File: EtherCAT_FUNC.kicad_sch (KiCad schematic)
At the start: 31 parts, among them J1 axt430124, J10 Conn_01x02, J11 Conn_01x02, J12 Conn_01x02, J13 Conn_01x02, J14 Conn_01x02, J15 Conn_01x02, J16 Conn_01x02, J2 Conn_01x02, J3 Conn_01x02, J4 Conn_01x04, J8 Conn_01x03, J9 Conn_01x02, U6 ESDS314

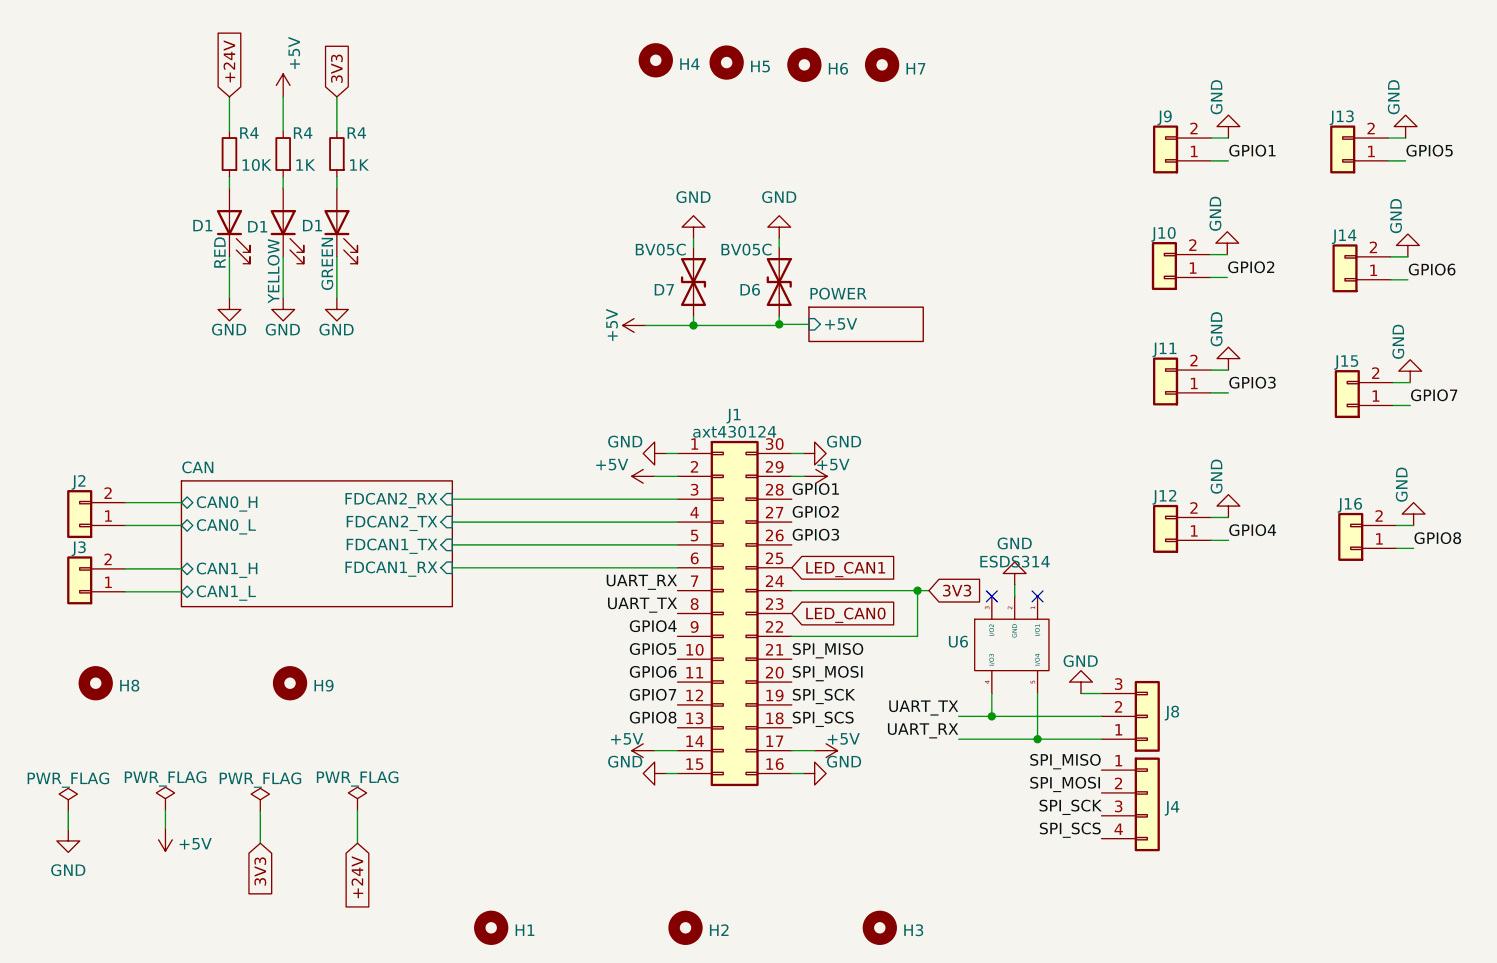
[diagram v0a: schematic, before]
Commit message: Official version
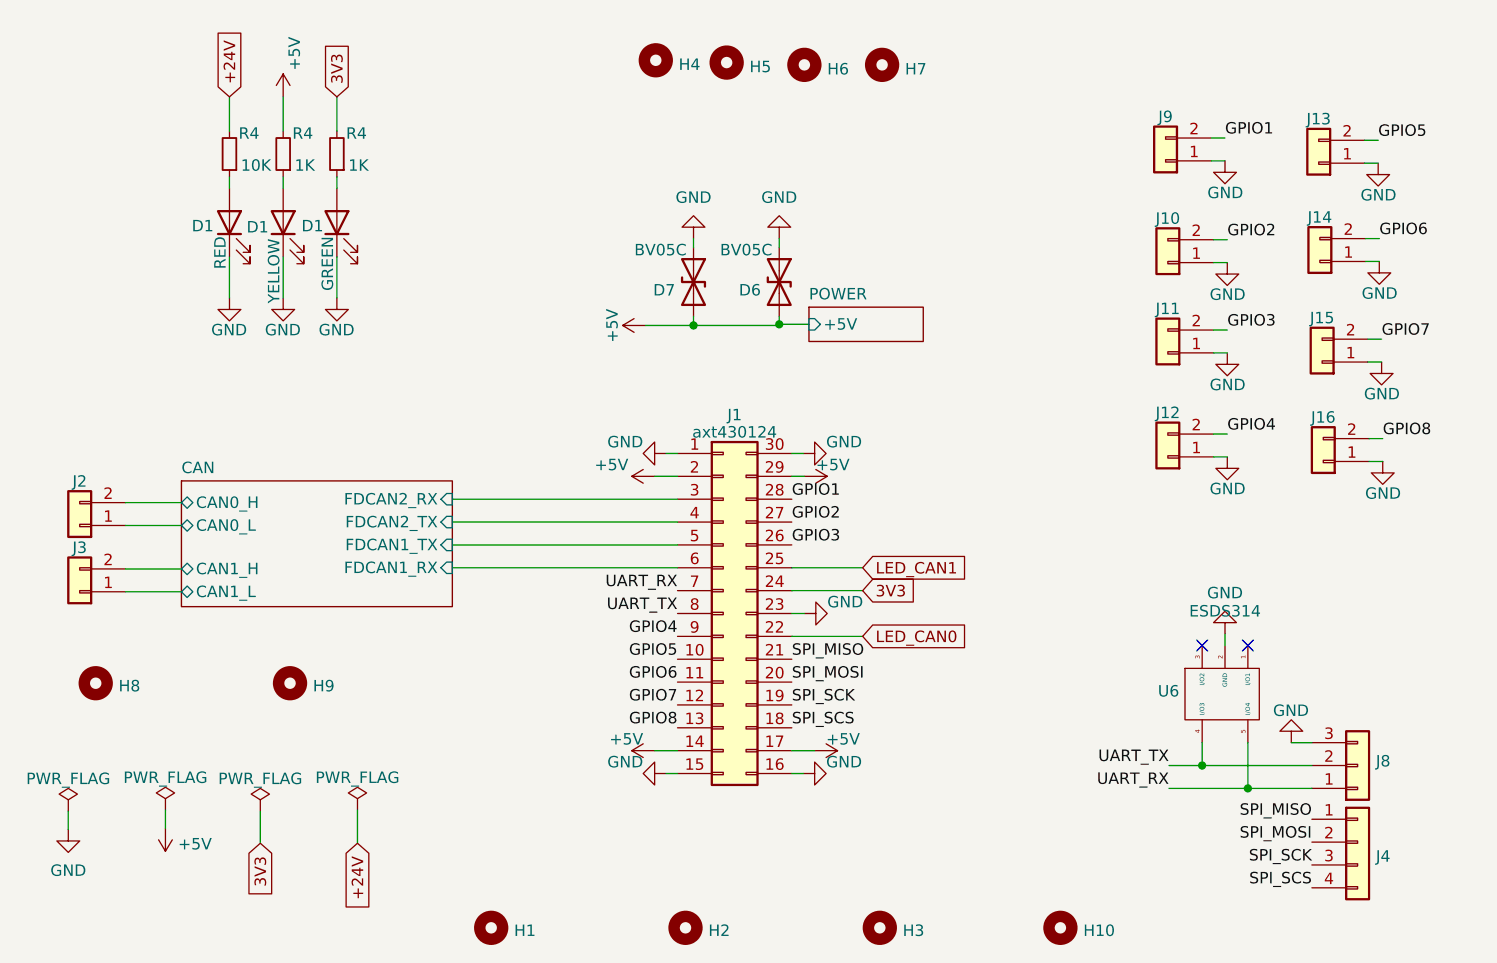
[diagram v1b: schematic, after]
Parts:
- added H10: MountingHole, EXTRA IC:M1.6, symbol Mechanical:MountingHole
- H4, H5, H6, H7: footprint EXTRA IC:M1.6 -> EXTRA IC:M2_HOLE
- H8, H9: footprint EXTRA IC:M2 -> EXTRA IC:M2_noHOLE
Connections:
- net 3V3: no longer J1.22
- net GND: now also J1.23, J10.1 (Pin_1), J11.1 (Pin_1), J12.1 (Pin_1), J13.1 (Pin_1), J14.1 (Pin_1), J15.1 (Pin_1), J16.1 (Pin_1), J9.1 (Pin_1); no longer J10.2 (Pin_2), J11.2 (Pin_2), J12.2 (Pin_2), J13.2 (Pin_2), J14.2 (Pin_2), J15.2 (Pin_2), J16.2 (Pin_2), J9.2 (Pin_2)
- net GPIO1: now also J9.2 (Pin_2); no longer J9.1 (Pin_1)
- net GPIO2: now also J10.2 (Pin_2); no longer J10.1 (Pin_1)
- net GPIO3: now also J11.2 (Pin_2); no longer J11.1 (Pin_1)
- net GPIO4: now also J12.2 (Pin_2); no longer J12.1 (Pin_1)
- net GPIO5: now also J13.2 (Pin_2); no longer J13.1 (Pin_1)
- net GPIO6: now also J14.2 (Pin_2); no longer J14.1 (Pin_1)
- net GPIO7: now also J15.2 (Pin_2); no longer J15.1 (Pin_1)
- net GPIO8: now also J16.2 (Pin_2); no longer J16.1 (Pin_1)
- net LED_CAN0: now also J1.22; no longer J1.23
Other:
- moved on the sheet: J4, J8, U6
